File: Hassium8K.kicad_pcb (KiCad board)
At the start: 2 copper layers, 59.9 x 63 mm, 52 parts, among them J1 Conn_01x04_Pin, J2 Conn_01x04_Pin, J3 Conn_01x04_Pin, J4 Conn_01x04_Pin, J5 C596731, J6 C596731, J7 Conn_01x08_Pin, SW1 SW_DPST_x2, SW2 SW_DPST_x2, SW3 SW_DPST_x2, SW4 SW_DPST_x2, U1 STM32H723VGTx, U2 USB3300-EZK, U3 XC6206PxxxMR, U4 STM32F072CBTx, Y1 C5261152, Y2 C9002

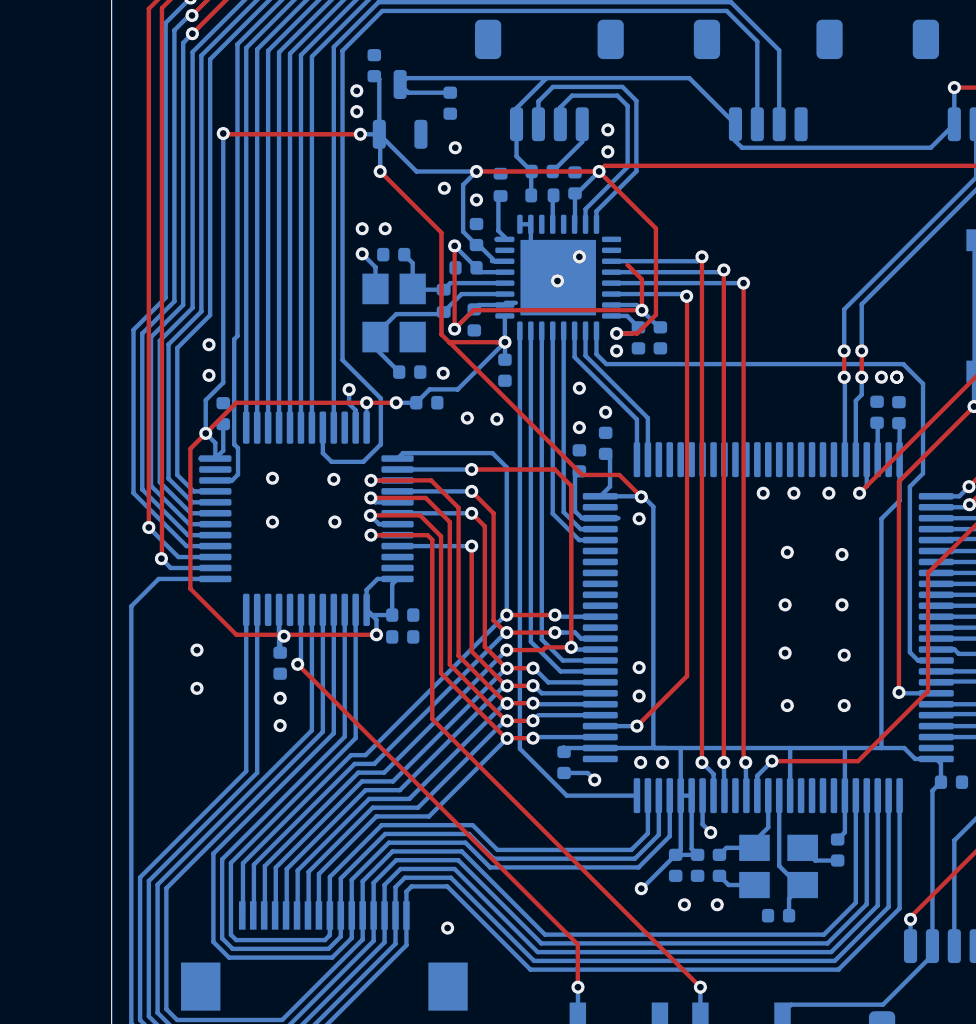
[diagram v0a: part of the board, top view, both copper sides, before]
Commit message: Add files via upload
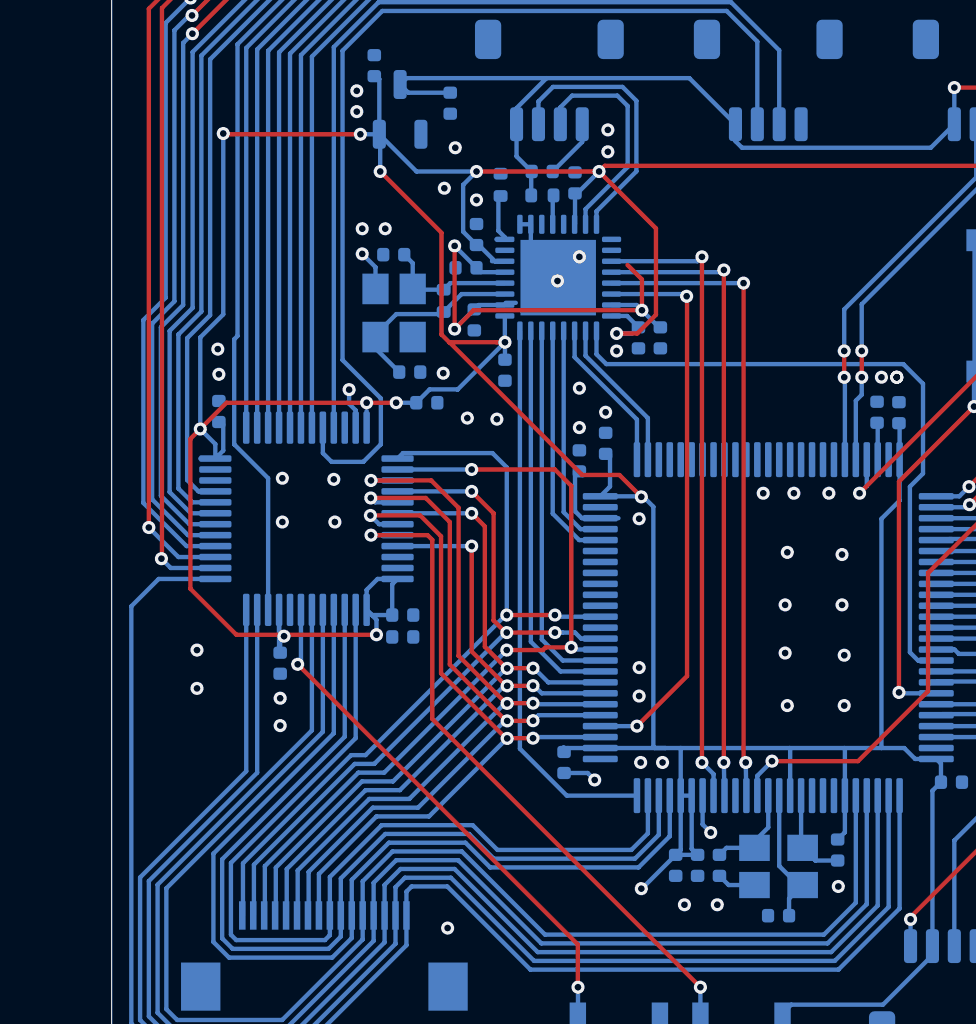
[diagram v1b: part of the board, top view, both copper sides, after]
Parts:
- moved C25 0.22 mm to (563.4, 434.0)
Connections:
- U4 pad 10: unconnected-(U4-PA0-Pad10) -> COL7-1
- U4 pad 22: COL7-1 -> unconnected-(U4-PB11-Pad22)
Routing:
- net COL7-1: track 160.6 -> 166.2 mm
- net GND: track 31.1 -> 33.5 mm, vias 55 -> 56
- net COL8-1: track 164.3 -> 163.8 mm
